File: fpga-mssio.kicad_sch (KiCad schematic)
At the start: 15 parts, among them U1 MPFS250T-FCVG484, U30 NTS0102_XSON

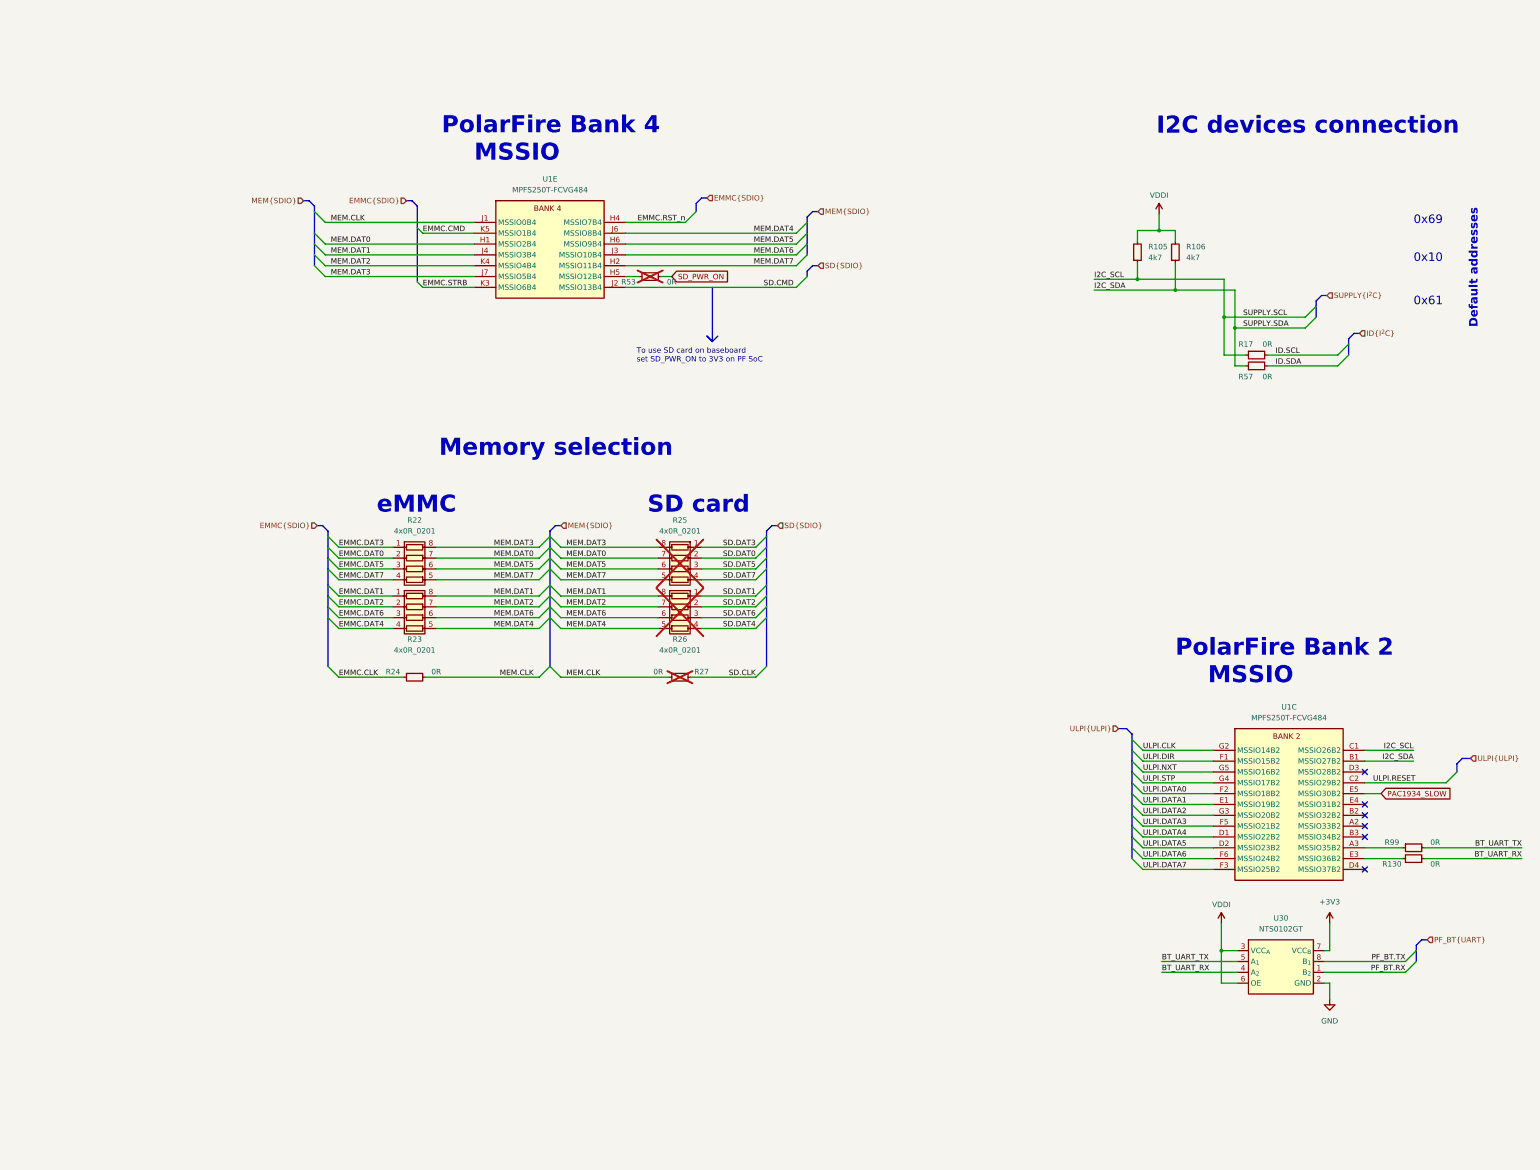
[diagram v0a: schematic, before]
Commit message: [#57422] Finishing touches
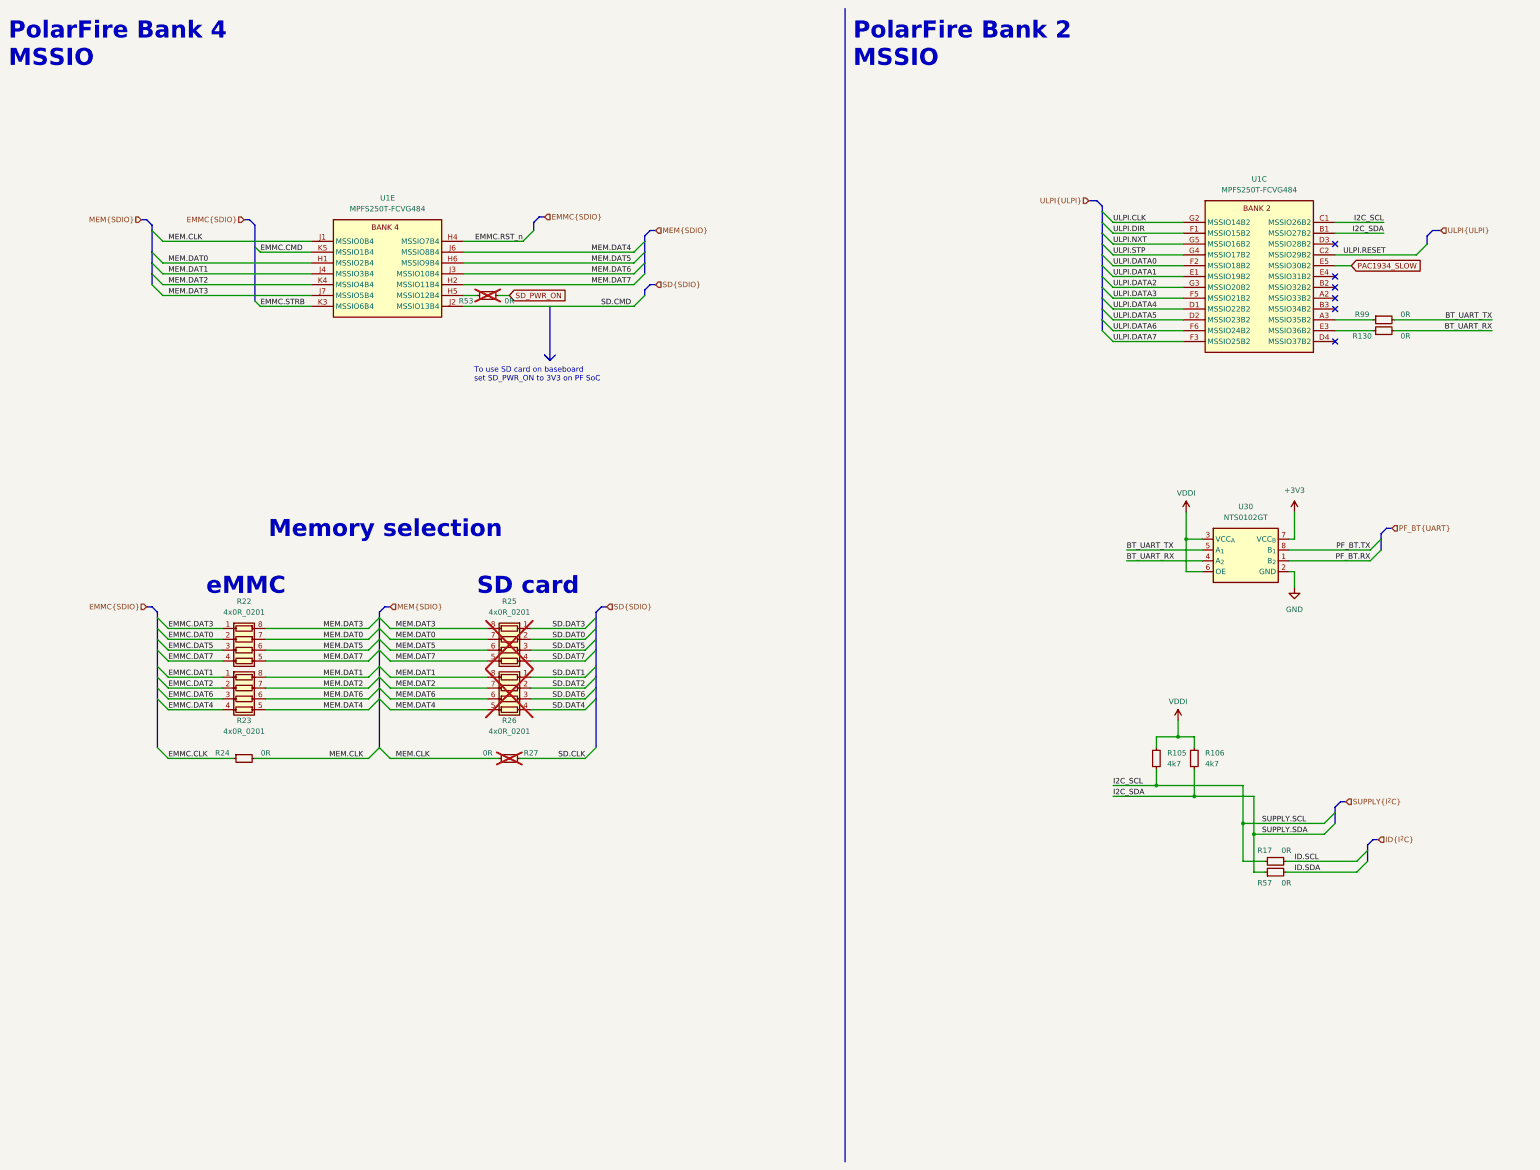
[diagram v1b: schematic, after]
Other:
- note removed: "0x10"
- note removed: "0x61"
- note removed: "0x69"
- note removed: "Default addresses"
- note removed: "I2C devices connection"
- moved on the sheet: R105, R106, R130, R17, R22, R23, R24, R25, R26, R27, R53, R57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
